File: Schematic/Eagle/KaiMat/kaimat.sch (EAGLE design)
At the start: 53 parts, among them X1 OPAMP

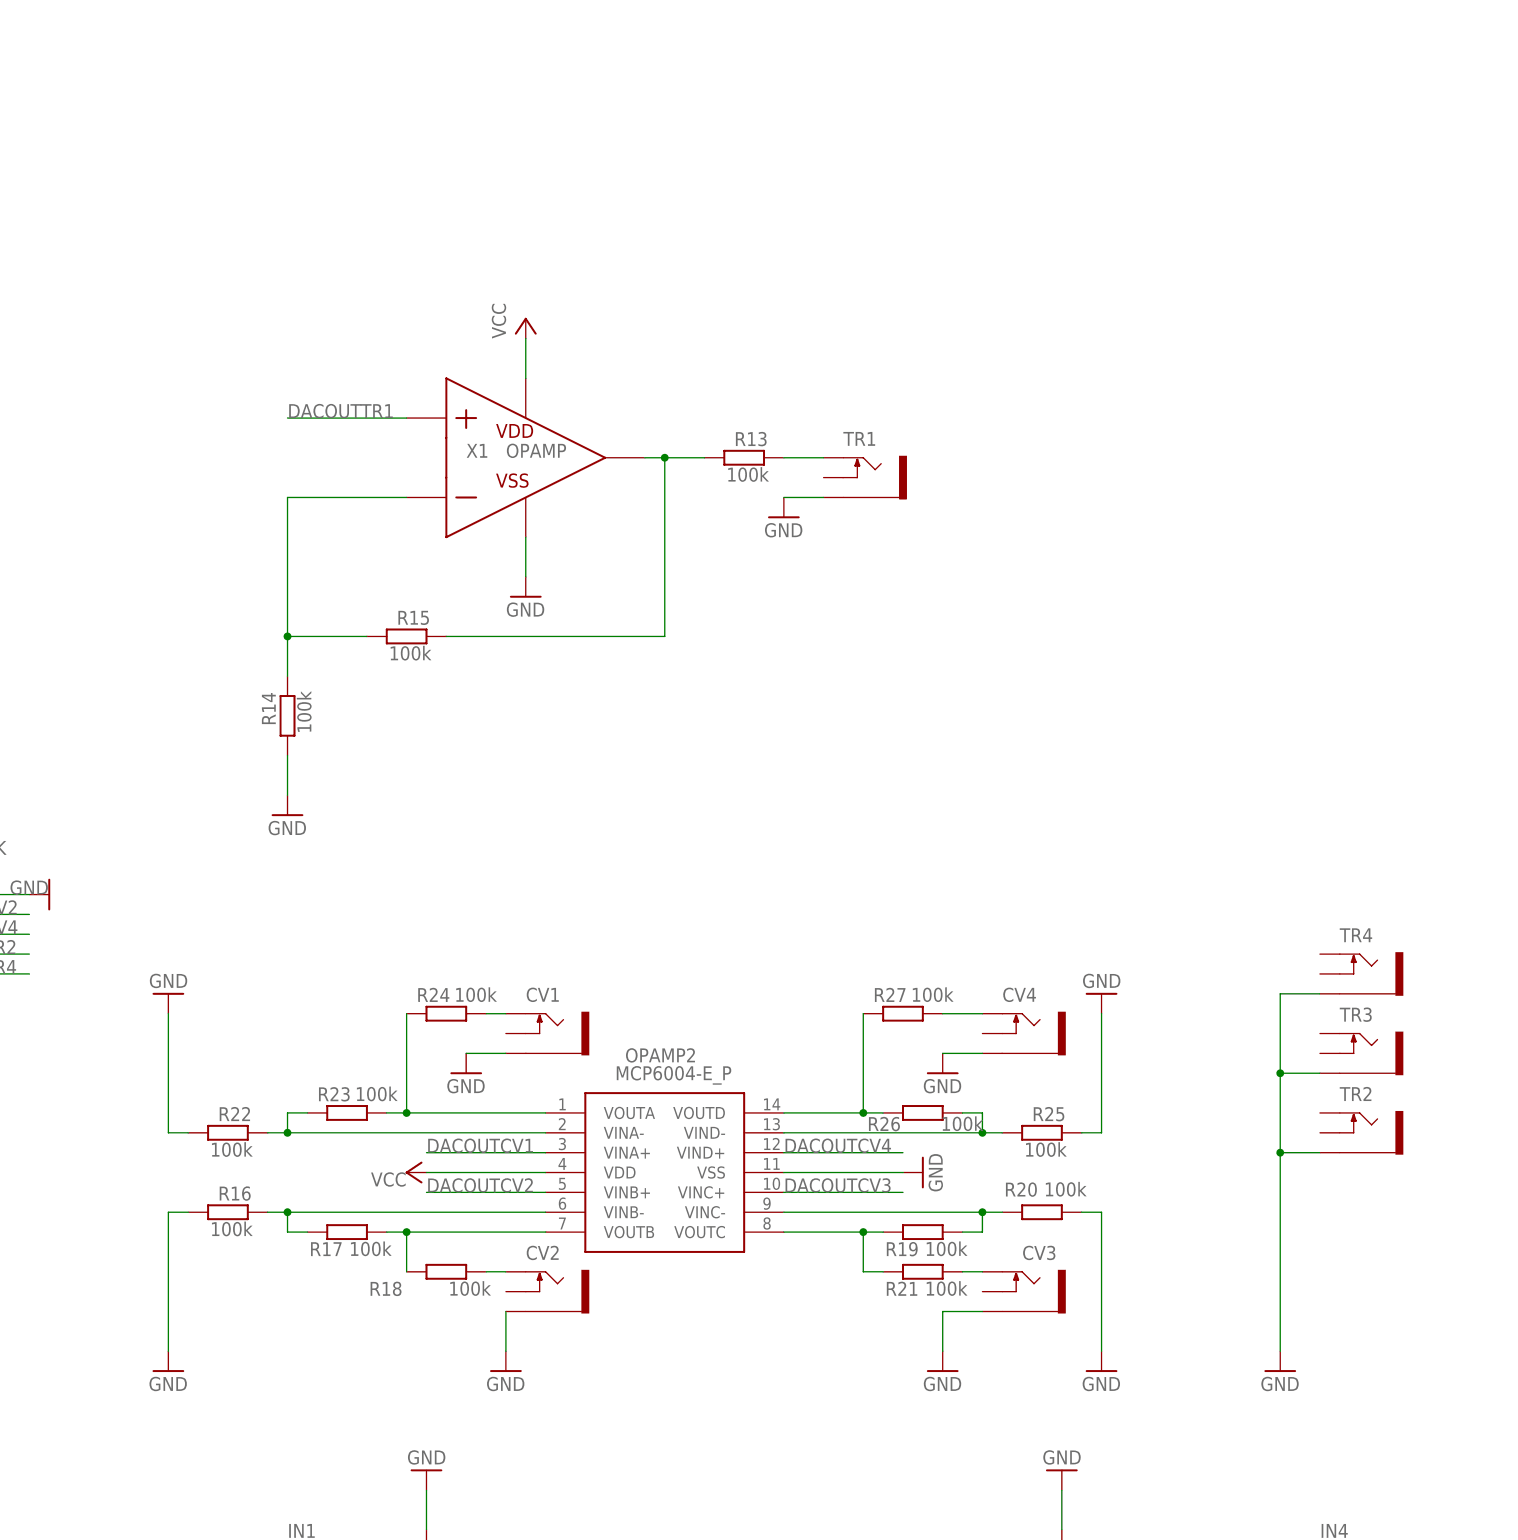
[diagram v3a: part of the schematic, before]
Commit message: updated circuit and pcb
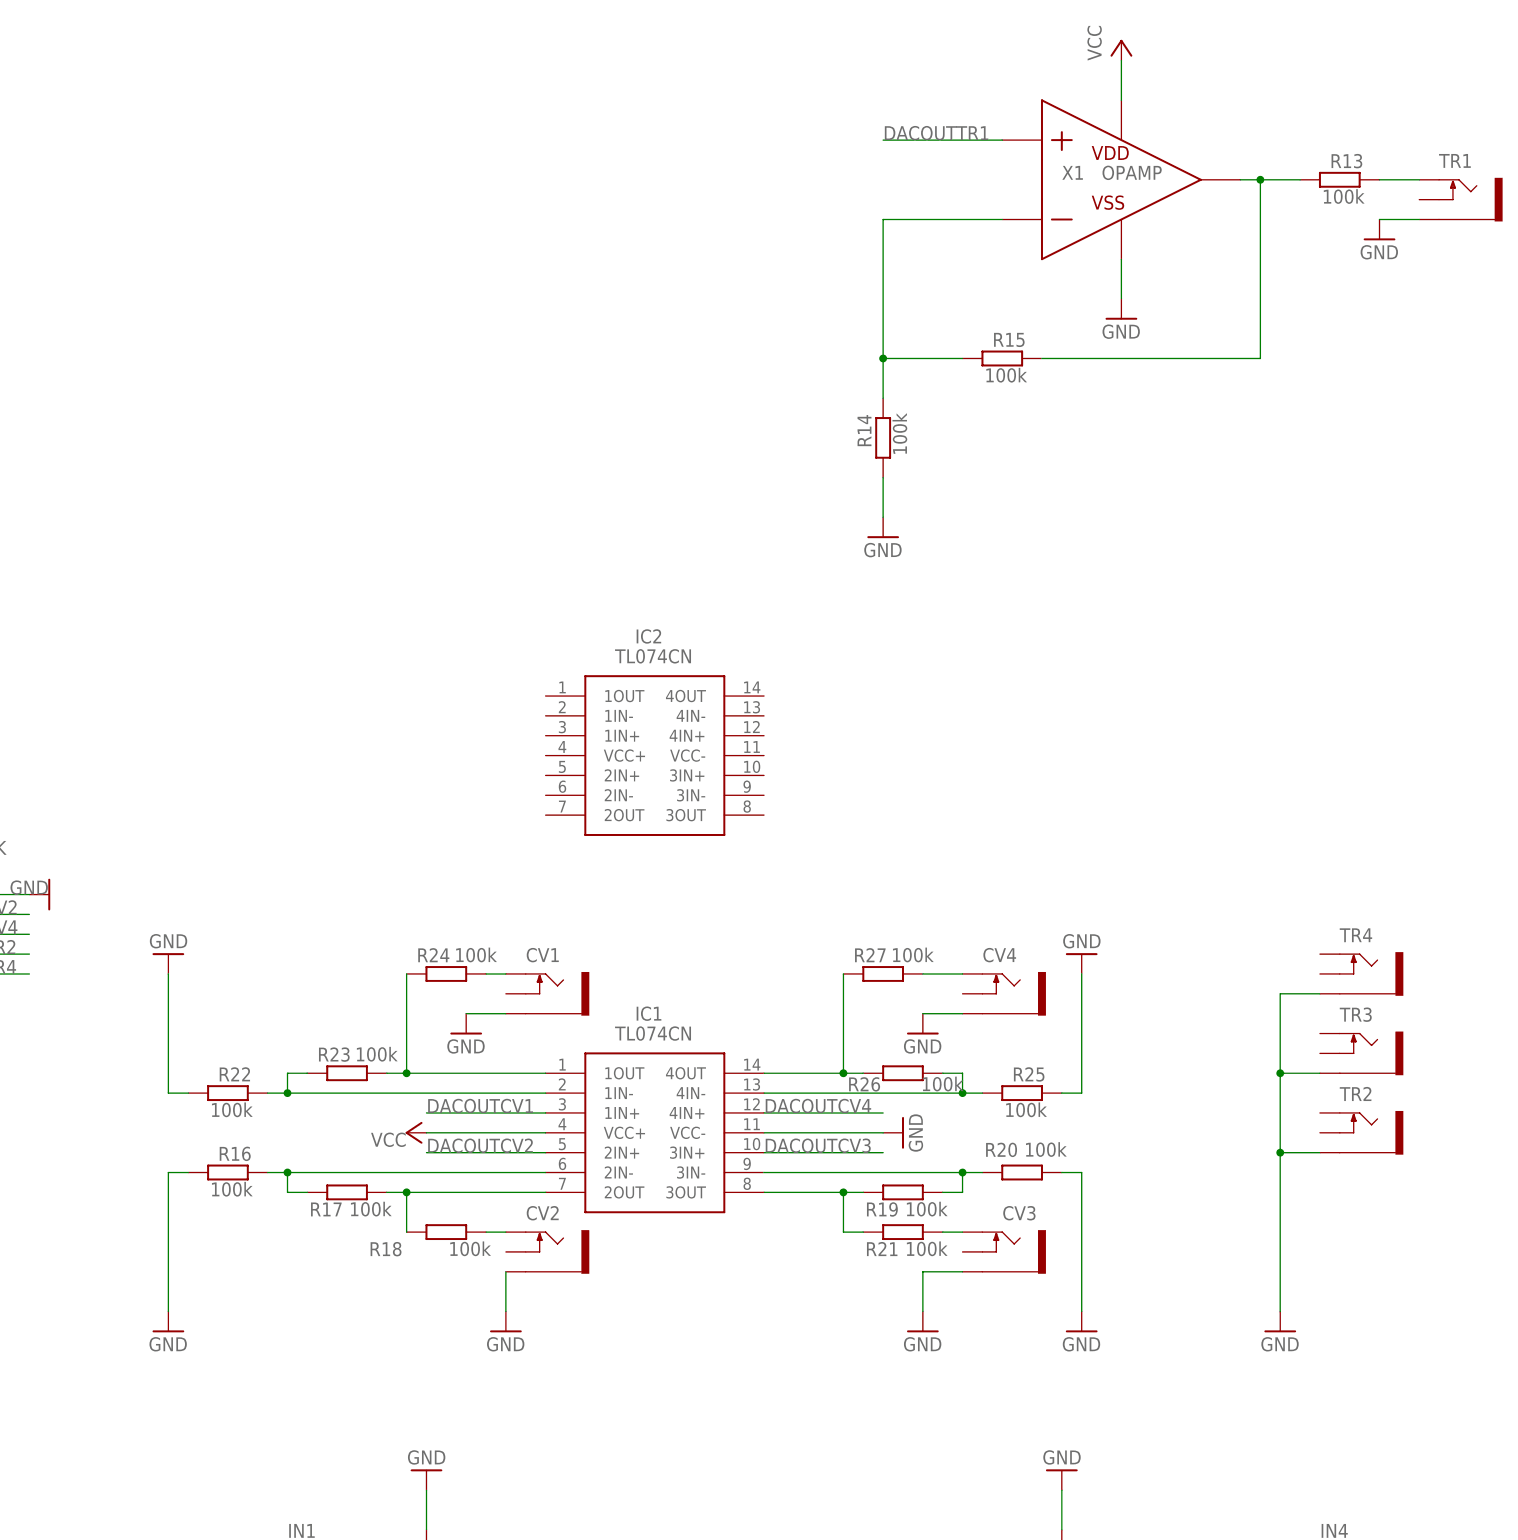
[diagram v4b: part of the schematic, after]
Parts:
- removed OPAMP2: MCP6004-E_P, mcp6004-e_p:MCP6004-E_P
- added IC1, IC2: TL074CN, TL074CN:TL074CN
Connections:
- net DACOUTCV1: now also IC1.1IN+; no longer OPAMP2.VINA+
- net DACOUTCV2: now also IC1.2IN+; no longer OPAMP2.VINB+
- net DACOUTCV3: now also IC1.3IN+; no longer OPAMP2.VINC+
- net DACOUTCV4: now also IC1.4IN+; no longer OPAMP2.VIND+
- net GND: now also IC1.VCC-; no longer OPAMP2.VSS
- net N$17: now also IC1.2IN-; no longer OPAMP2.VINB-
- net N$2: now also IC1.2OUT; no longer OPAMP2.VOUTB
- net N$21: now also IC1.3OUT; no longer OPAMP2.VOUTC
- net N$22: now also IC1.3IN-; no longer OPAMP2.VINC-
- net N$23: now also IC1.1IN-; no longer OPAMP2.VINA-
- net N$24: now also IC1.1OUT; no longer OPAMP2.VOUTA
- net N$26: now also IC1.4IN-; no longer OPAMP2.VIND-
- net N$27: now also IC1.4OUT; no longer OPAMP2.VOUTD
- net VCC: now also IC1.VCC+; no longer OPAMP2.VDD
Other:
- moved on the sheet: CV1, CV2, CV3, CV4, R13, R14, R15, R16, R17, R18, R19, R20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

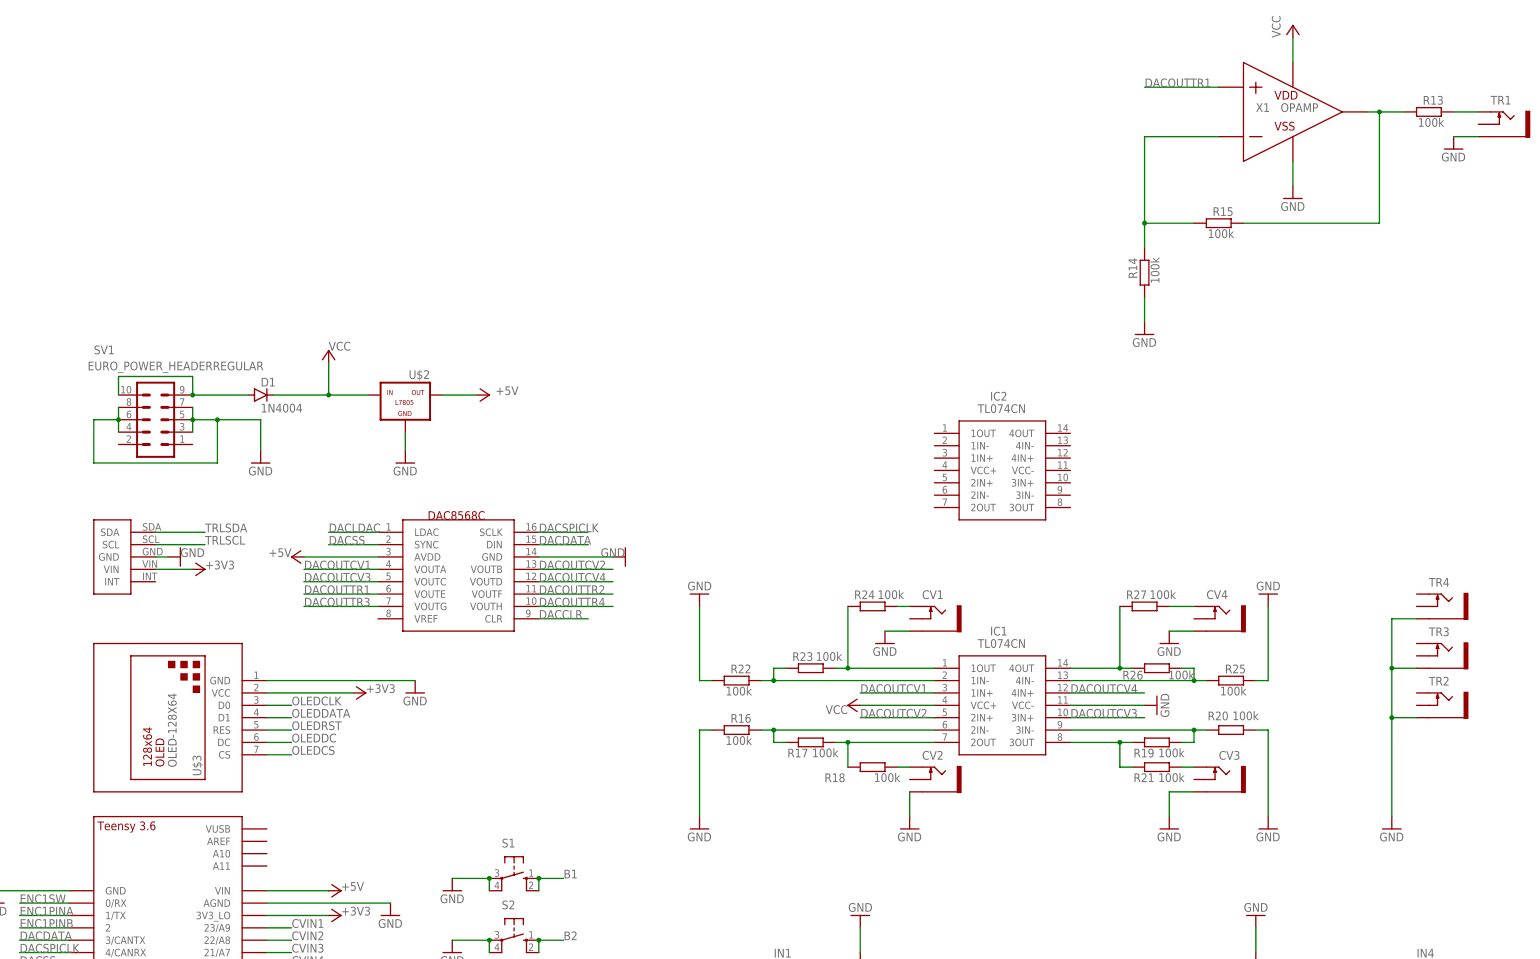
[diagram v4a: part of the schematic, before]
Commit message: finished schematic
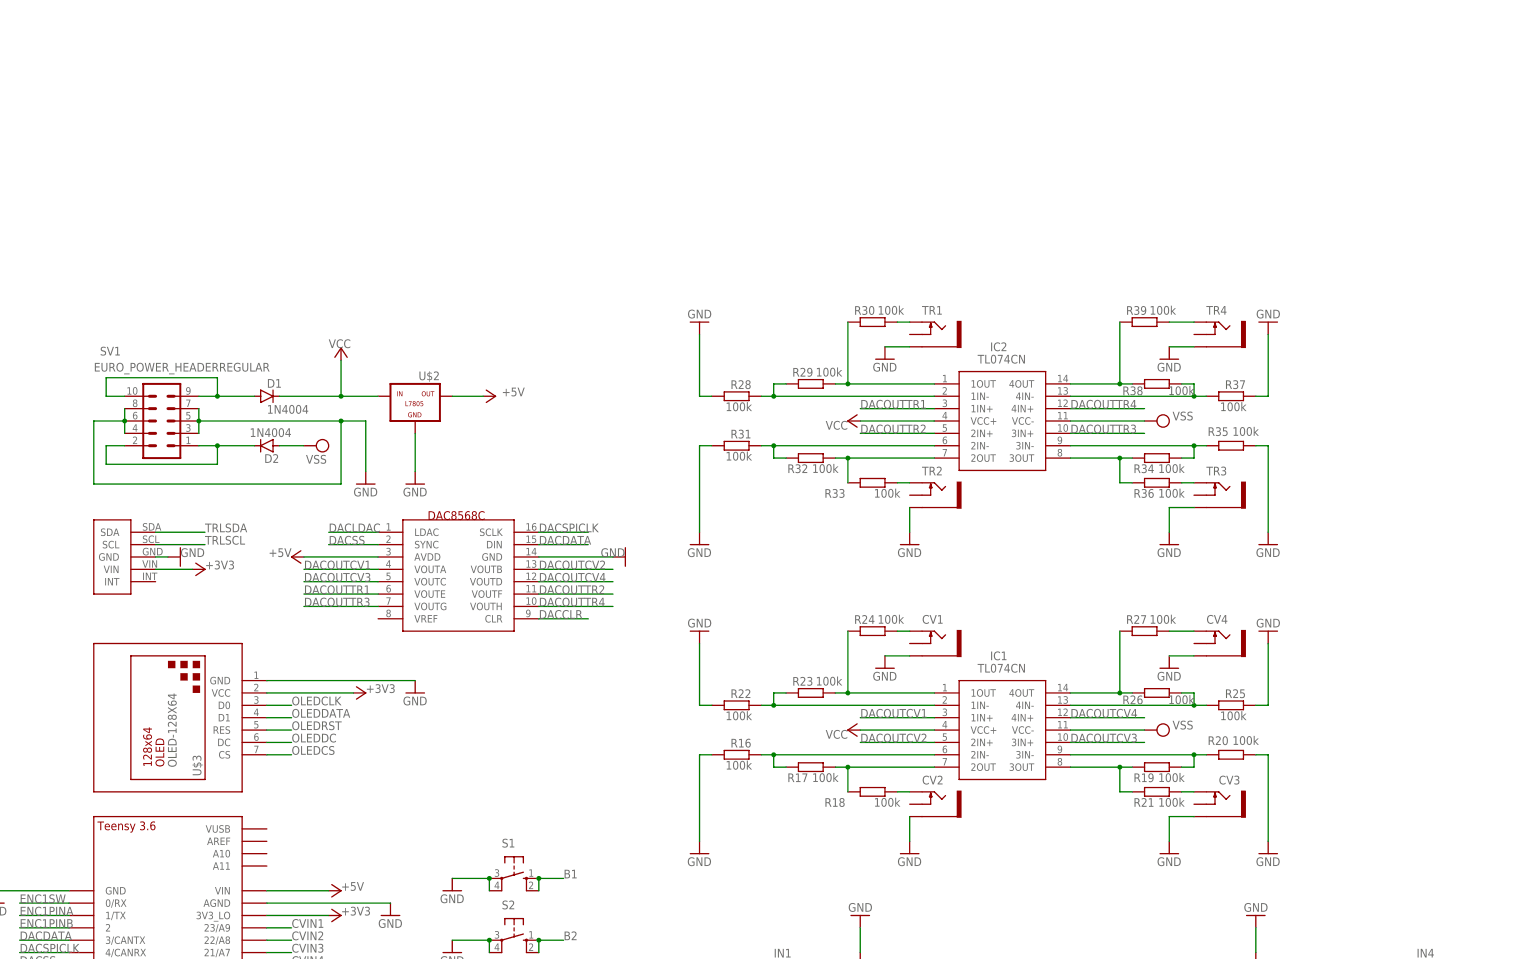
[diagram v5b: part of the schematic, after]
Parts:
- removed R13, R14, R15: 100k, MusicThingModular:RESISTOR7MM
- removed X1: OPAMP, ngspice-simulation:OPAMP
- added D2: 1N4004, diode:1N4004
- added R28, R29, R30, R31, R32, R33, R34, R35, R36, R37, R38, R39: 100k, MusicThingModular:RESISTOR7MM
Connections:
- removed net N$10: R14.2, R15.1, X1.N
- removed net N$8: R13.1, R15.2, X1.VOUT
- new net N$29: D2.C, SV1.1, SV1.2
- new net N$30: IC2.1IN-, R28.2, R29.1
- new net N$31: IC2.1OUT, R29.2, R30.1
- new net N$32: IC2.2IN-, R31.2, R32.1
- new net N$33: R30.2, TR1.TIP
- new net N$34: R33.2, TR2.TIP
- new net N$35: IC2.3IN-, R34.2, R35.1
- new net N$36: R36.2, TR3.TIP
- new net N$37: IC2.3OUT, R34.1, R36.1
- new net N$38: IC2.4IN-, R37.1, R38.2
- new net N$39: IC2.4OUT, R38.1, R39.1
- new net N$40: R39.2, TR4.TIP
- new net VSS: D2.A, IC1.VCC-, IC2.VCC-
- net DACOUTTR1: now also IC2.1IN+; no longer X1.P
- net DACOUTTR2: now also IC2.2IN+
- net DACOUTTR3: now also IC2.3IN+
- net DACOUTTR4: now also IC2.4IN+
- net GND: now also R28.1, R31.1, R35.2, R37.2; no longer IC1.VCC-, R14.1, X1.VSS
- net N$7: now also IC2.2OUT, R32.2, R33.1; no longer R13.2, TR1.TIP
- net VCC: now also IC2.VCC+; no longer X1.VDD
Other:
- moved on the sheet: CV1, CV2, CV3, CV4, D1, IC1, IC2, R16, R17, R18, R19, R20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
